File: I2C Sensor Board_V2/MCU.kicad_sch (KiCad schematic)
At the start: 51 parts, among them IC1 MCP6006UT-E_OT, J1 Conn_02x03_Odd_Even, J2 Conn_01x04_MountingPin, J3 Barrel_Jack_Switch, J4 Conn_02x03_Odd_Even, J5 USB_B, J7 Conn_01x04_MountingPin, Q4 PMOS, SW1 SW_DIP_x01, U1 ATmega328P-A, U2 AP62300TWU, U3 CH340G, Y1 16 MHz, Y4 12 MHz

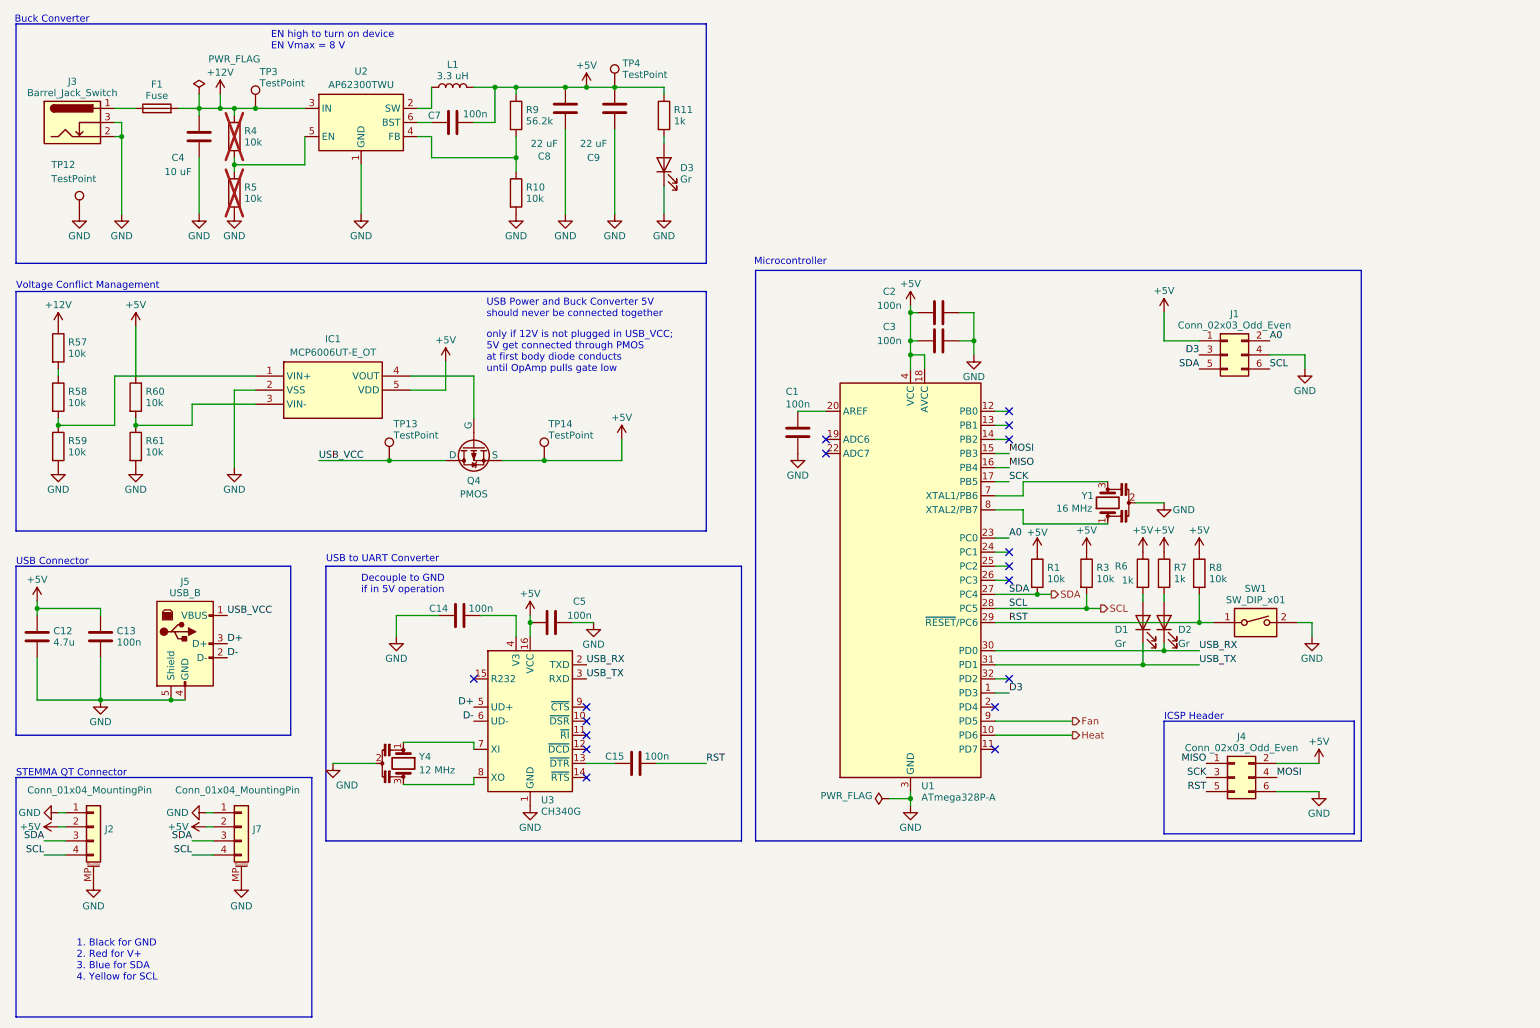
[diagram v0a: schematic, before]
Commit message: Add files via upload
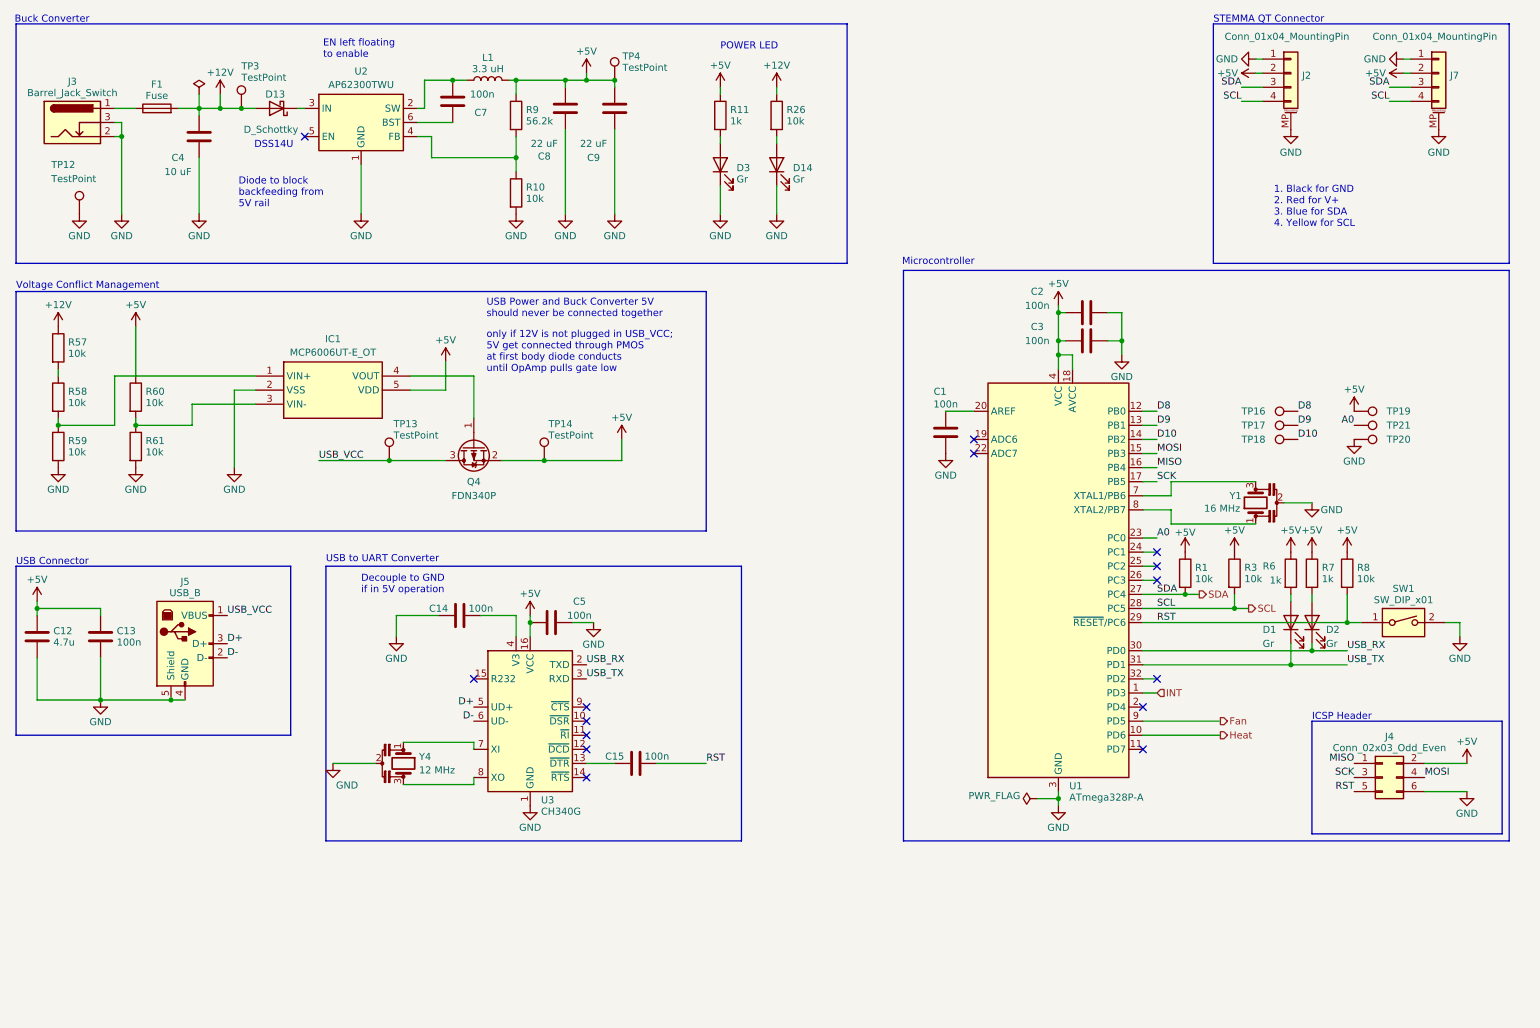
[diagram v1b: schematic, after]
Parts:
- removed J1: Conn_02x03_Odd_Even, Connector_PinHeader_2.54mm:PinHeader_2x03_P2.54mm_Vertical, symbol Connector_Generic:Conn_02x03_Odd_Even
- removed Q4: PMOS, Created:SOT95P237X112-3N, symbol Simulation_SPICE:PMOS
- removed R4, R5: 10k, Resistor_SMD:R_0805_2012Metric_Pad1.20x1.40mm_HandSolder, symbol Device:R
- added D13: D_Schottky, Diode_SMD:D_SOD-123F, symbol Device:D_Schottky
- added D14: Gr, LED_SMD:LED_0805_2012Metric_Pad1.15x1.40mm_HandSolder, symbol Device:LED
- added Q4: FDN340P, Package_TO_SOT_SMD:SOT-23, symbol Transistor_FET:FDN340P
- added R26: 10k, Resistor_SMD:R_0805_2012Metric_Pad1.20x1.40mm_HandSolder, symbol Device:R
- added TP16, TP17, TP18, TP19, TP20, TP21: TestPoint, TestPoint:TestPoint_THTPad_D1.5mm_Drill0.7mm, symbol Connector:TestPoint
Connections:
- net +12V: now also D13.2 (A), R26.1; no longer U2.3 (IN)
- net +5V: now also Q4.2 (S), TP19.1; no longer C7.2
- net A0: now also TP21.1
- net GND: now also D14.1 (K), TP20.1
- net USB_VCC: now also Q4.3 (D)
- net at L1.1, U2.2 (SW): now also C7.2
- net at IC1.4 (VOUT): now also Q4.1 (G)
- net D8: now reaches U1.12 (PB0)
- net D8: now also TP16.1
- net D9: now reaches U1.13 (PB1)
- net D9: now also TP17.1
- net D10: now reaches U1.14 (PB2)
- net D10: now also TP18.1
- net D3 renamed INT
- new net: D13.1 (K), U2.3 (IN)
- new net: D14.2 (A), R26.2
- no-connect marks 17 -> 15
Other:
- note added: "DSS14U"
- note added: "Diode to block backfeeding from 5V rail"
- note added: "EN left floating to enable"
- note added: "POWER LED"
- note removed: "EN high to turn on device EN Vmax = 8 V"
- moved on the sheet: C1, C2, C3, C7, D1, D2, D3, J2, J4, J7, L1, R1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
